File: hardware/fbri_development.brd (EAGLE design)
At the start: 95 parts, among them IC3 TLV70033DCK, J1 AAA_HOLDER, U1 SAM_D20E, U2 SI4060, U3 MAX1947, U4 ANTENOVA_GPS_M10382, U5 S25FS-S, U6 STM32F_48PIN, Y1 8MHz

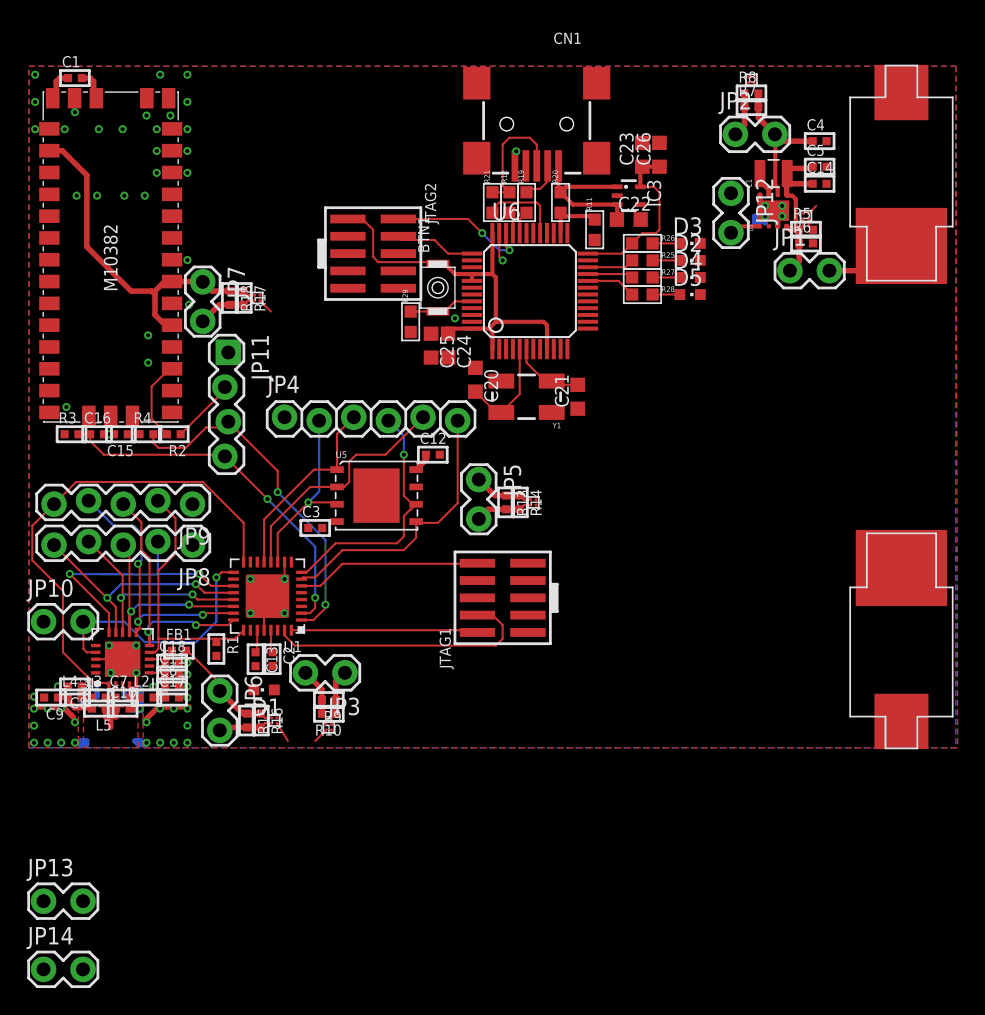
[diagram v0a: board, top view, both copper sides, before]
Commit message: Before trying Direct Tie Tx/Rx
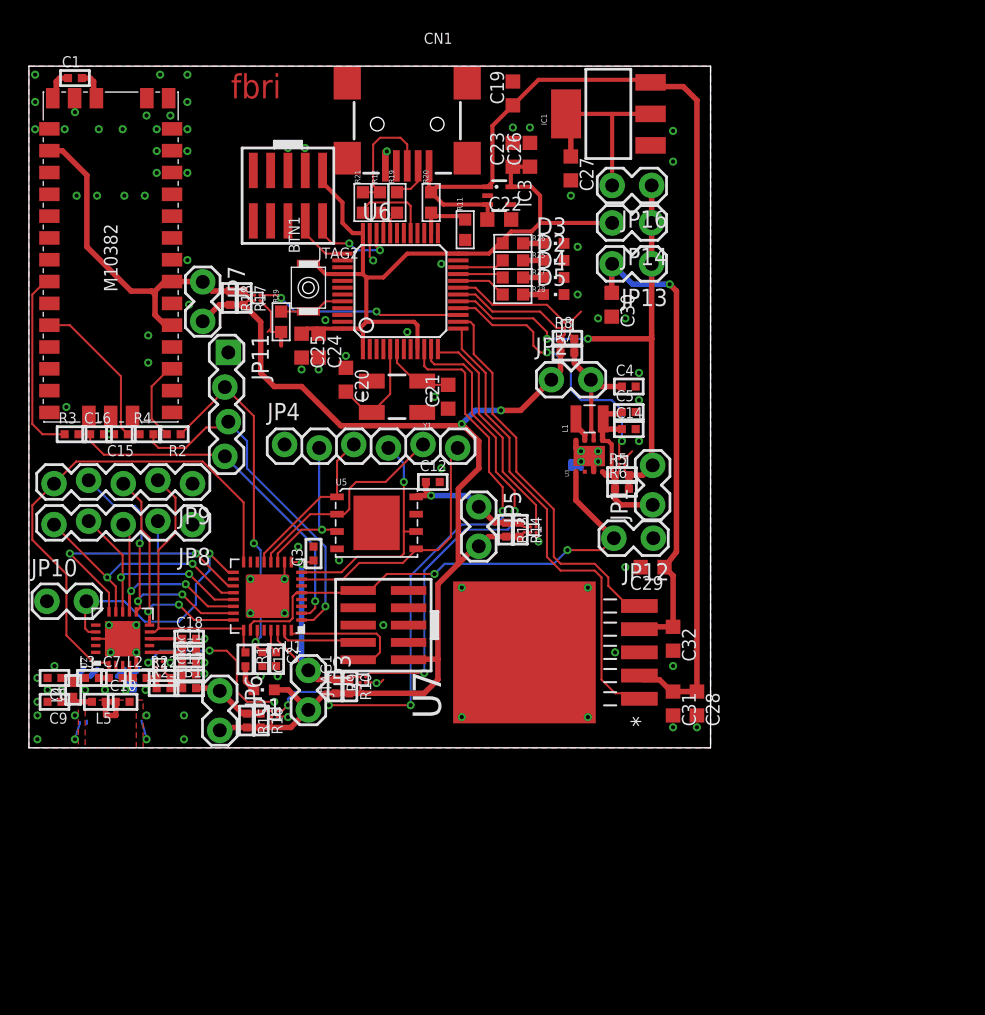
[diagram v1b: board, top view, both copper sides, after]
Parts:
- removed J1: AAA_HOLDER, fbri:AAA
- added C19: 4.7µF, resistor:C0603K
- added C27, C28, C29, C30: 10µF, resistor:C0603K
- added C31, C32: 100pF, resistor:C0603K
- added IC1: (no value), SparkFun:SOT223
- added JP16: (no value), SparkFun:1X02_LOCK
- added R22, R23: 1Ω, microbuilder_v3:_0402
- added U$99: INA216, fbri:WCSP-4
- added U7: LP38501TS-ADJ/NOPB, LP38501TS-ADJ:TO170P1435X457-6N
- moved JP14 70.4 mm to (45.5, 38.5), turned to 180 degrees
- moved JP13 64.4 mm to (45.5, 35.5), turned to 180 degrees
- moved JP12 25.8 mm to (45.6, 15.4), turned to 180 degrees
- moved C14 22.8 mm to (44.0, 23.4)
- moved C4 22.8 mm to (44.0, 26.5)
- moved C5 22.8 mm to (44.0, 24.6)
- moved JP2 22.5 mm to (38.5, 27.0)
- moved L1 22.5 mm to (41.1, 24.1)
- moved R5 22.5 mm to (43.5, 20.0)
- moved R6 22.5 mm to (43.5, 19.0)
- moved R7 22.5 mm to (39.5, 29.0)
- moved R8 22.5 mm to (39.5, 30.0)
- moved U$2 22.5 mm to (43.5, 21.0)
- moved U$5 22.5 mm to (39.5, 31.0)
- moved U3 22.5 mm to (41.1, 21.4)
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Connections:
- removed net N$1: U6.10
- removed net N$5: JP1.2, JP13.1, JP14.1, R5.2, R6.2, U$2.A1
- removed net PWR_BR: U6.19
- new net 1.2VREG_OUT: C27.1, IC1.2, IC1.4, JP16.2
- new net ADJ_REG_EN: U6.13, U7.1
- new net ADJ_REG_OUT: C29.1, C30.1, C32.1, JP13.2, U7.4
- new net ADJ_REG_SWITCHING: U6.14, U7.5
- new net I_PA: U$99.B2
- new net I_STEPUP_IN: U$2.B2, U6.16
- new net I_STEPUP_OUT: U$5.B2, U6.19
- new net I_VDD_GPS: U$62.B2, U6.15
- new net I_VDD_MEM: U$48.B2, U6.12
- new net I_VDD_RADIO: U$60.B2, U6.10
- new net I_VDD_SAMD20: U$30.B2, U6.11
- new net VDD_PA: L2.2, R22.1, R23.1, U$99.A2
- new net VDD_STEPUP: JP1.2, JP13.1, JP14.1, JP16.1, R5.2, R6.2, U$2.A1, U6.17
- net 1.2V: no longer J1.+2, JP13.2
- net 1.8V: now also U6.18
- net 3.3V: now also JP14.2; no longer U6.41
- net 5.0V: now also C19.1, C28.1, C31.1, IC1.3, U7.2
- net GND: now also C19.2, C27.2, C28.2, C29.2, C30.2, C31.2, C32.2, IC1.1, U$99.B1, U7.3, U7.6; no longer J1.-1, J1.-2
- net RADIO_VDD: now also R22.2, R23.2, U$99.A1; no longer L2.2
- net RESETN: now also U1.5; no longer U1.15, U1.6
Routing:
- net 1.8V: track 20.4 -> 98.8 mm, vias 0 -> 2
- net 5.0V: track 11.9 -> 81.7 mm
- net I_VDD_RADIO: track 0.00 -> 45.5 mm, vias 0 -> 4
- net VDD_STEPUP: track 0.00 -> 40.1 mm, vias 0 -> 2
- net I_VDD_SAMD20: track 0.00 -> 36.5 mm, vias 0 -> 2
- net ADJ_REG_OUT: track 0.00 -> 35.4 mm, vias 0 -> 1
- net ADJ_REG_EN: track 0.00 -> 35.1 mm
- net ADJ_REG_SWITCHING: track 0.00 -> 28.8 mm
- net RESETN: track 15.9 -> 36.7 mm, vias 0 -> 2
- net TIME_1KHZ: track 6.47 -> 26.9 mm, vias 0 -> 2
- net I_STEPUP_IN: track 0.00 -> 20.2 mm, vias 0 -> 2
- net I_VDD_MEM: track 0.00 -> 16.9 mm
- net I_VDD_GPS: track 0.00 -> 15.2 mm, vias 0 -> 2
- net 1.2VREG_OUT: track 0.00 -> 14.8 mm
- net SWDCLK: track 20.0 -> 6.06 mm
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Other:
- board outline added: 50 x 50 mm
- board text added: "!IRQ"
- board text added: "!SEL"
- board text added: "Board"
- board text added: "Devlopment"
- board text added: "GPS UART"
- board text added: "HFCLK"
- board text added: "Radio SPI"
- board text removed: "HF_CLK"
- board text removed: "NIRQ"
- board text removed: "NSEL"
